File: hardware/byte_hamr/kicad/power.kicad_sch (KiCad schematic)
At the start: 49 parts, among them U1 LFE5U-85F-8BG381I, U3 TLV62569DBV, U4 TLV62569DBV, U5 TLV62569DBV

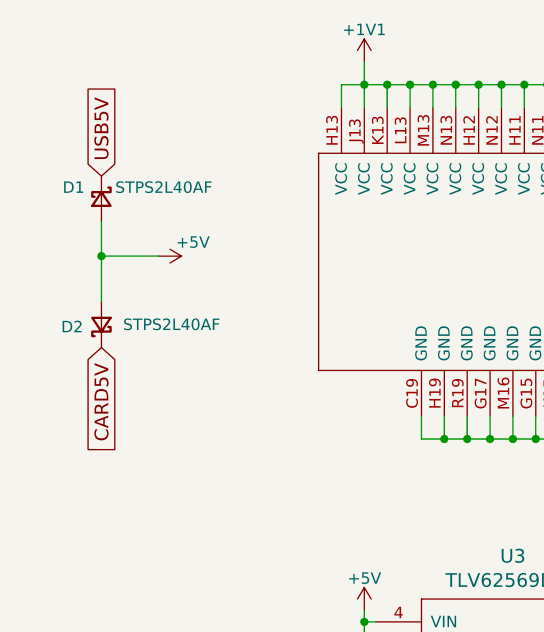
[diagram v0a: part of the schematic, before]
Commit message: Rev. 2
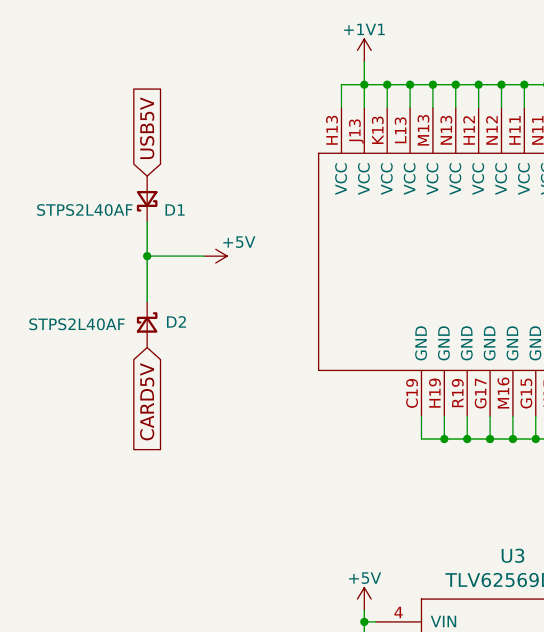
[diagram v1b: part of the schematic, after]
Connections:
- net +5V: now also D1.1 (K), D2.1 (K); no longer D1.2 (A), D2.2 (A)
- net CARD5V: now also D2.2 (A); no longer D2.1 (K)
- net USB5V: now also D1.2 (A); no longer D1.1 (K)
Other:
- moved on the sheet: D1, D2
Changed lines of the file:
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@@
 	)
 	(junction
-		(at 24.13 48.26)
+		(at 29.21 48.26)
 		(diameter 0)
 		(color 0 0 0 0)
@@
 	(wire
 		(pts
-			(xy 24.13 48.26) (xy 24.13 53.34)
+			(xy 29.21 48.26) (xy 29.21 53.34)
 		)
 		(stroke
@@
 	(wire
 		(pts
-			(xy 24.13 44.45) (xy 24.13 48.26)
+			(xy 29.21 44.45) (xy 29.21 48.26)
 		)
 		(stroke
@@
 	(wire
 		(pts
-			(xy 24.13 48.26) (xy 30.48 48.26)
+			(xy 29.21 48.26) (xy 35.56 48.26)
 		)
 		(stroke
@@
 	(global_label "CARD5V"
 		(shape input)
-		(at 24.13 58.42 270)
+		(at 29.21 58.42 270)
 		(effects
 			(font
@@
 		)
 		(property "Intersheetrefs" "${INTERSHEET_REFS}"
-			(at 24.13 58.42 0)
+			(at 29.21 58.42 0)
 			(effects
 				(font
@@
 	(global_label "USB5V"
 		(shape input)
-		(at 24.13 39.37 90)
+		(at 29.21 39.37 90)
 		(effects
 			(font
@@
 		)
 		(property "Intersheetrefs" "${INTERSHEET_REFS}"
-			(at 24.13 39.37 90)
+			(at 29.21 39.37 90)
 			(effects
 				(font
@@
 	(symbol
 		(lib_id "Device:D_Schottky_Small")
-		(at 24.13 41.91 270)
+		(at 29.21 41.91 90)
 		(unit 1)
 		(exclude_from_sim no)
@@
 		(dnp no)
 		(property "Reference" "D1"
-			(at 19.812 40.64 90)
+			(at 33.528 43.18 90)
 			(effects
 				(font
@@
 		)
 		(property "Value" "STPS2L40AF"
-			(at 25.654 40.64 90)
+			(at 27.686 43.18 90)
 			(effects
 				(font
@@
 		)
 		(property "Footprint" "Diode_SMD:D_SMA"
-			(at 24.13 41.91 90)
+			(at 29.21 41.91 90)
 			(effects
 				(font
@@
 		)
 		(property "Datasheet" ""
-			(at 24.13 41.91 90)
+			(at 29.21 41.91 90)
 			(effects
 				(font
@@
 		)
 		(property "Description" ""
-			(at 24.13 41.91 0)
+			(at 29.21 41.91 0)
 			(effects
 				(font
@@
 		)
 		(property "MNF1_URL" "www.st.com"
-			(at 24.13 41.91 0)
+			(at 29.21 41.91 0)
 			(effects
 				(font
@@
 		)
 		(property "MPN" "STPS2L30AF"
-			(at 24.13 41.91 0)
+			(at 29.21 41.91 0)
 			(effects
 				(font
@@
 		)
 		(property "Mouser" "511-STPS2L40AF"
-			(at 24.13 41.91 0)
+			(at 29.21 41.91 0)
 			(effects
 				(font
@@
 		)
 		(property "Digikey" "497-12310-1-ND"
-			(at 24.13 41.91 0)
+			(at 29.21 41.91 0)
 			(effects
 				(font
@@
 		)
 		(property "Newark" "69AH2828"
-			(at 24.13 41.91 0)
+			(at 29.21 41.91 0)
 			(effects
 				(font
@@
 		)
 		(property "AvnetEU" "STPS2L30AF"
-			(at 24.13 41.91 0)
+			(at 29.21 41.91 0)
 			(effects
 				(font
@@
 		)
 		(property "LCSC" "C111630"
-			(at 24.13 41.91 0)
+			(at 29.21 41.91 0)
 			(effects
 				(font
@@
 		)
 		(property "price100_AvnetEU" "0.22121$"
-			(at 24.13 41.91 0)
+			(at 29.21 41.91 0)
 			(effects
 				(font
@@
 		)
 		(property "Koncar" "FV008"
-			(at 24.13 41.91 0)
+			(at 29.21 41.91 0)
 			(effects
 				(font
@@
 	(symbol
 		(lib_id "power:+5V")
-		(at 30.48 48.26 270)
+		(at 35.56 48.26 270)
 		(unit 1)
 		(exclude_from_sim no)
@@
 		(dnp no)
 		(property "Reference" "#PWR01"
-			(at 26.67 48.26 0)
+			(at 31.75 48.26 0)
 			(effects
 				(font
@@
 		)
 		(property "Value" "+5V"
-			(at 34.29 46.736 90)
+			(at 39.37 46.736 90)
 			(effects
 				(font
@@
 		)
 		(property "Footprint" ""
-			(at 30.48 48.26 0)
+			(at 35.56 48.26 0)
 			(effects
 				(font
@@
 		)
 		(property "Datasheet" ""
-			(at 30.48 48.26 0)
+			(at 35.56 48.26 0)
 			(effects
 				(font
@@
 		)
 		(property "Description" ""
-			(at 30.48 48.26 0)
+			(at 35.56 48.26 0)
 			(effects
 				(font
@@
 	(symbol
 		(lib_id "Device:D_Schottky_Small")
-		(at 24.13 55.88 90)
+		(at 29.21 55.88 270)
 		(unit 1)
 		(exclude_from_sim no)
@@
 		(dnp no)
 		(property "Reference" "D2"
-			(at 22.098 56.134 90)
+			(at 31.242 55.626 90)
 			(effects
 				(font
@@
 		)
 		(property "Value" "STPS2L40AF"
-			(at 37.338 55.88 90)
+			(at 16.002 55.88 90)
 			(effects
 				(font
@@
 		)
 		(property "Footprint" "Diode_SMD:D_SMA"
-			(at 24.13 55.88 90)
+			(at 29.21 55.88 90)
 			(effects
 				(font
@@
 		)
 		(property "Datasheet" ""
-			(at 24.13 55.88 90)
+			(at 29.21 55.88 90)
 			(effects
 				(font
@@
 		)
 		(property "Description" ""
-			(at 24.13 55.88 0)
+			(at 29.21 55.88 0)
 			(effects
 				(font
@@
 		)
 		(property "MNF1_URL" "www.st.com"
-			(at 24.13 55.88 0)
+			(at 29.21 55.88 0)
 			(effects
 				(font
@@
 		)
 		(property "MPN" "STPS2L30AF"
-			(at 24.13 55.88 0)
+			(at 29.21 55.88 0)
 			(effects
 				(font
@@
 		)
 		(property "Mouser" "511-STPS2L40AF"
-			(at 24.13 55.88 0)
+			(at 29.21 55.88 0)
 			(effects
 				(font
@@
 		)
 		(property "Digikey" "497-12310-1-ND"
-			(at 24.13 55.88 0)
+			(at 29.21 55.88 0)
 			(effects
 				(font
@@
 		)
 		(property "Newark" "69AH2828"
-			(at 24.13 55.88 0)
+			(at 29.21 55.88 0)
 			(effects
 				(font
@@
 		)
 		(property "AvnetEU" "STPS2L30AF"
-			(at 24.13 55.88 0)
+			(at 29.21 55.88 0)
 			(effects
 				(font
@@
 		)
 		(property "LCSC" "C111630"
-			(at 24.13 55.88 0)
+			(at 29.21 55.88 0)
 			(effects
 				(font
@@
 		)
 		(property "price100_AvnetEU" "0.22121$"
-			(at 24.13 55.88 0)
+			(at 29.21 55.88 0)
 			(effects
 				(font
@@
 		)
 		(property "Koncar" "FV008"
-			(at 24.13 55.88 0)
+			(at 29.21 55.88 0)
 			(effects
 				(font
